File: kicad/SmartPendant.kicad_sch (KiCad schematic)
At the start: 83 parts, among them P1 FPC 0.5MM 40P Pull type H2.0m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, P2 KH-FG0.5-H2.0-6PIN, Q1 SS8050_C2150, U1 74AHC2G125DP,125, U2 AMS1117-3.3, U3 MB85RC256VPNF

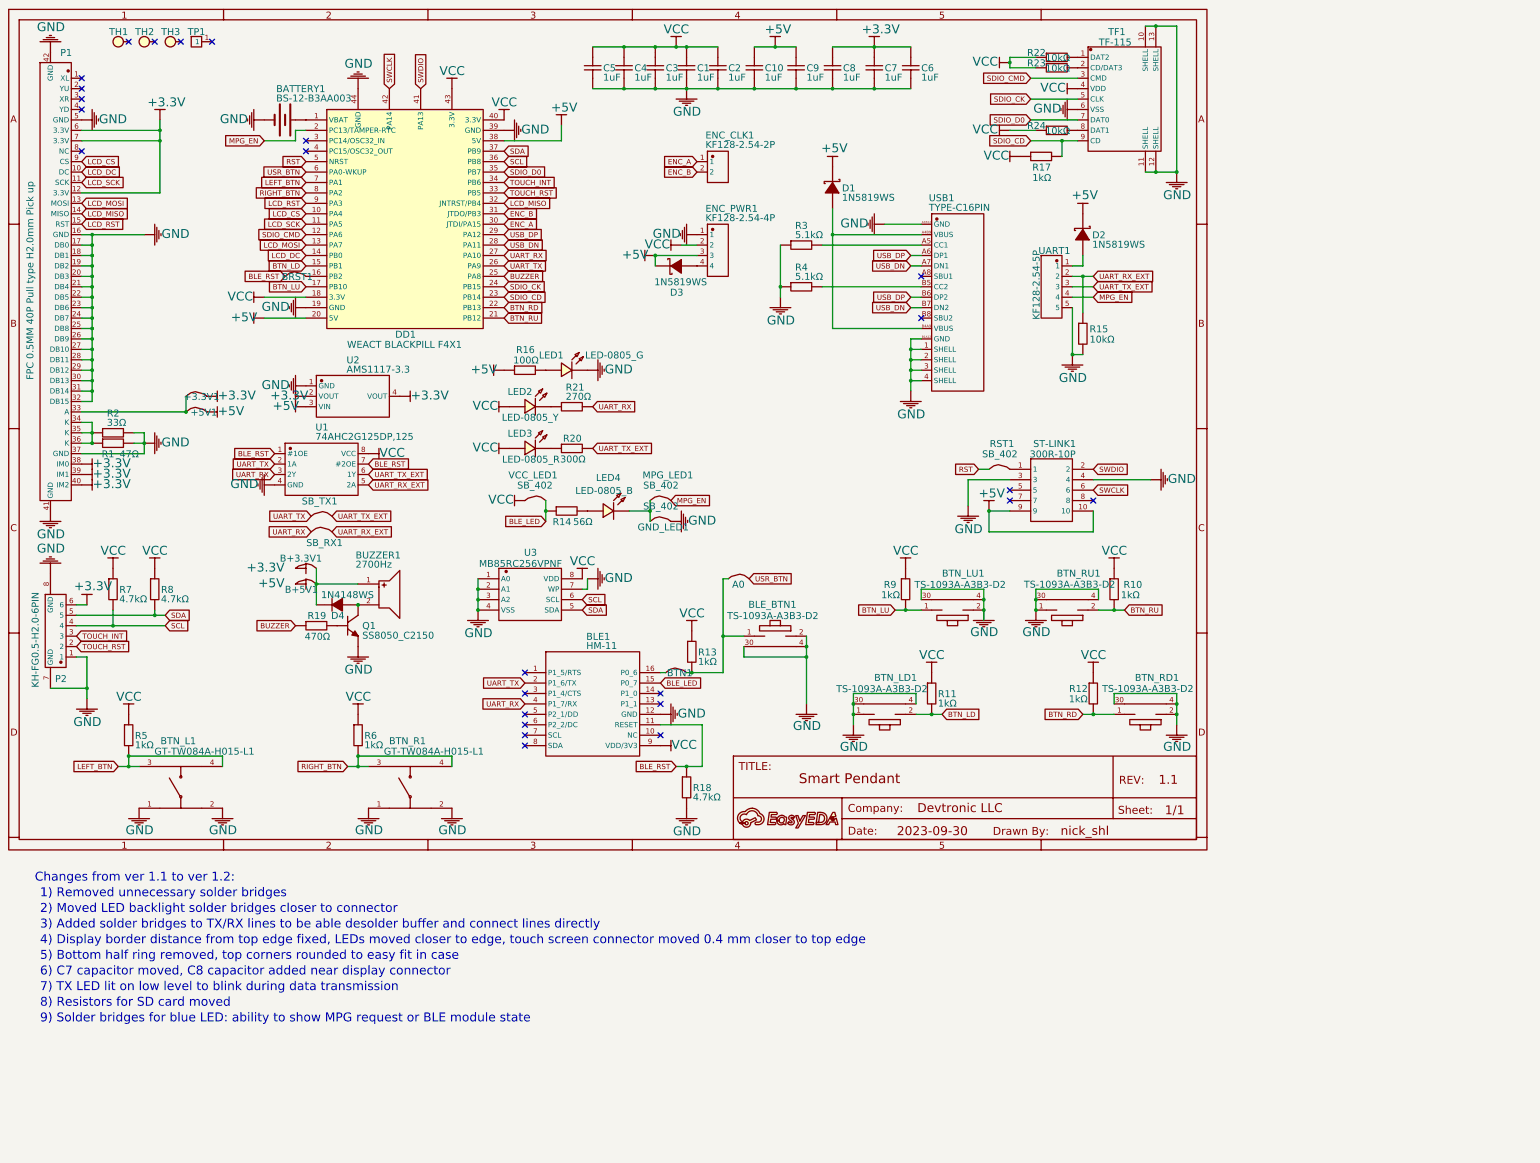
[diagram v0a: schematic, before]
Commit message: Fix cosmetics.
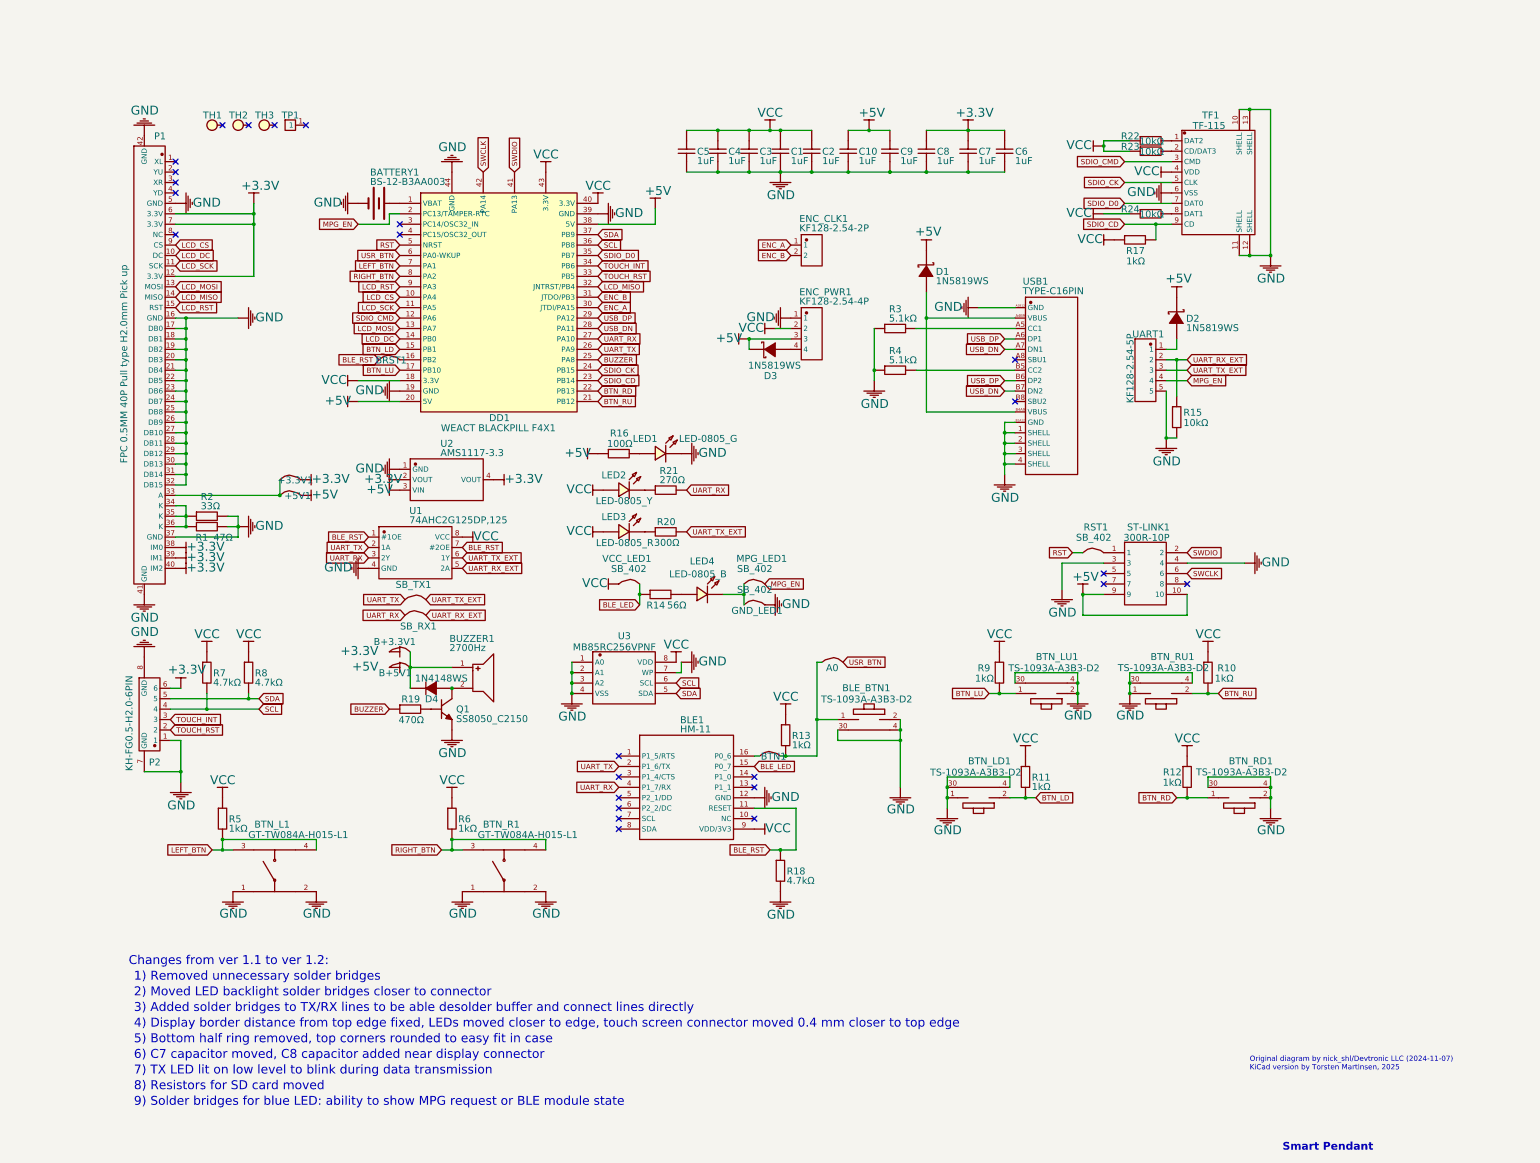
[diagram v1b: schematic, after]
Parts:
- removed A1: A, symbol Unknown_0_-806
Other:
- note added: "Original diagram by nick_shl/Devtronic LLC (2024-11-07) KiCad version by Torsten Martinsen, 2025"
- note added: "Smart Pendant"
- moved on the sheet: +3.3V1, +5V1, A0, B+3.3V1, B+5V1, BATTERY1, BLE1, BLE_BTN1, BRST1, BTN1, BTN_L1, BTN_LD1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
